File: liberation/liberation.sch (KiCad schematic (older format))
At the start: 21 parts, among them Q1 BC547BTA, Q2 BC547BTA, SW1 MHS122K, SW2 FSM4JAH, U1 NJU7223F33, U2 ESP32-WROOM-32D, U3 BME280

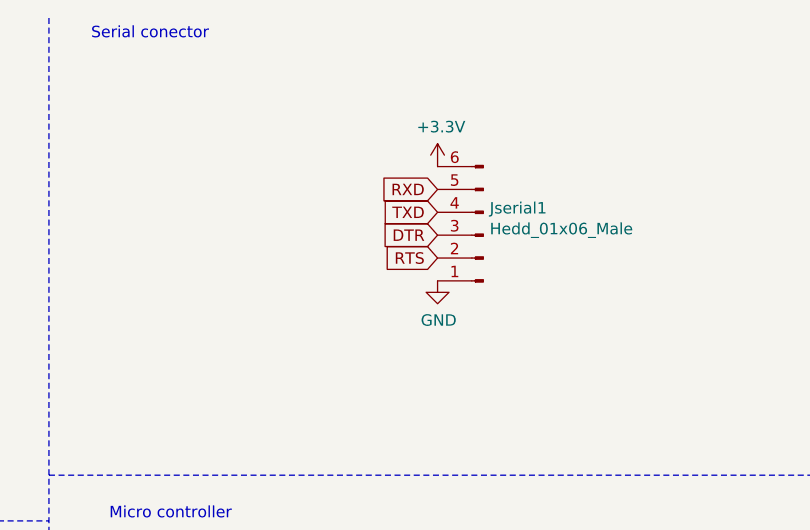
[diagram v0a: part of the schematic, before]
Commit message: Make PCB design (almost) complete :p
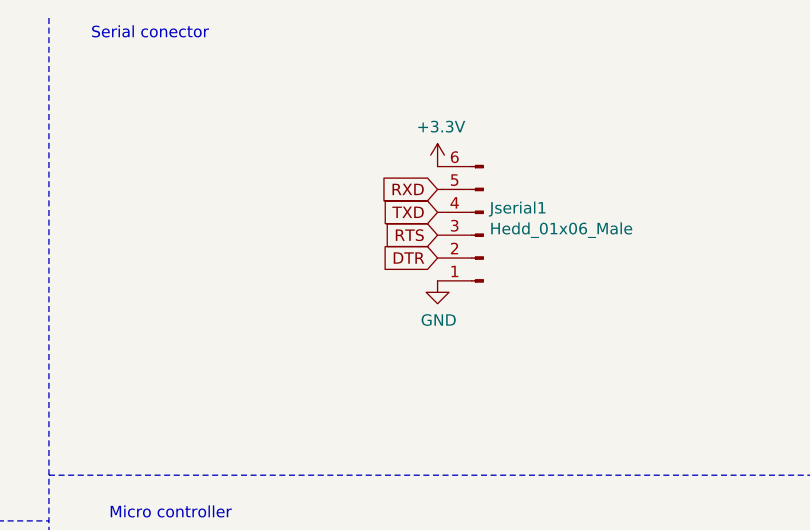
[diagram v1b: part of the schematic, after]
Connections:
- net DTR: now also Jserial1.2 (Pin_2); no longer Jserial1.3 (Pin_3)
- net RTS: now also Jserial1.3 (Pin_3); no longer Jserial1.2 (Pin_2)
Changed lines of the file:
@@
 Text GLabel 9250 1500 0    50   Input ~ 0
 TXD
+Text GLabel 9250 1700 0    50   Input ~ 0
+DTR
 Text GLabel 9250 1600 0    50   Input ~ 0
-DTR
-Text GLabel 9250 1700 0    50   Input ~ 0
 RTS
 $Comp
